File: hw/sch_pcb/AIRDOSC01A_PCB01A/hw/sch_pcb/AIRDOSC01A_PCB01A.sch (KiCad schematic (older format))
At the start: 22 parts, among them J1 HEADER_1x01, J2 HEADER_1x01, J3 HEADER_1x01, J4 HEADER_1x01, J5 CONN_2, J6 CONN_2, J7 HEADER_1x01, M1 HOLE, M2 HOLE, M3 HOLE, M4 HOLE, U1 ARRAYC-60035-4P-BGA, U2 MICROFC-60035-SMT-TR(1), U3 MICROFC-60035-SMT-TR(1)

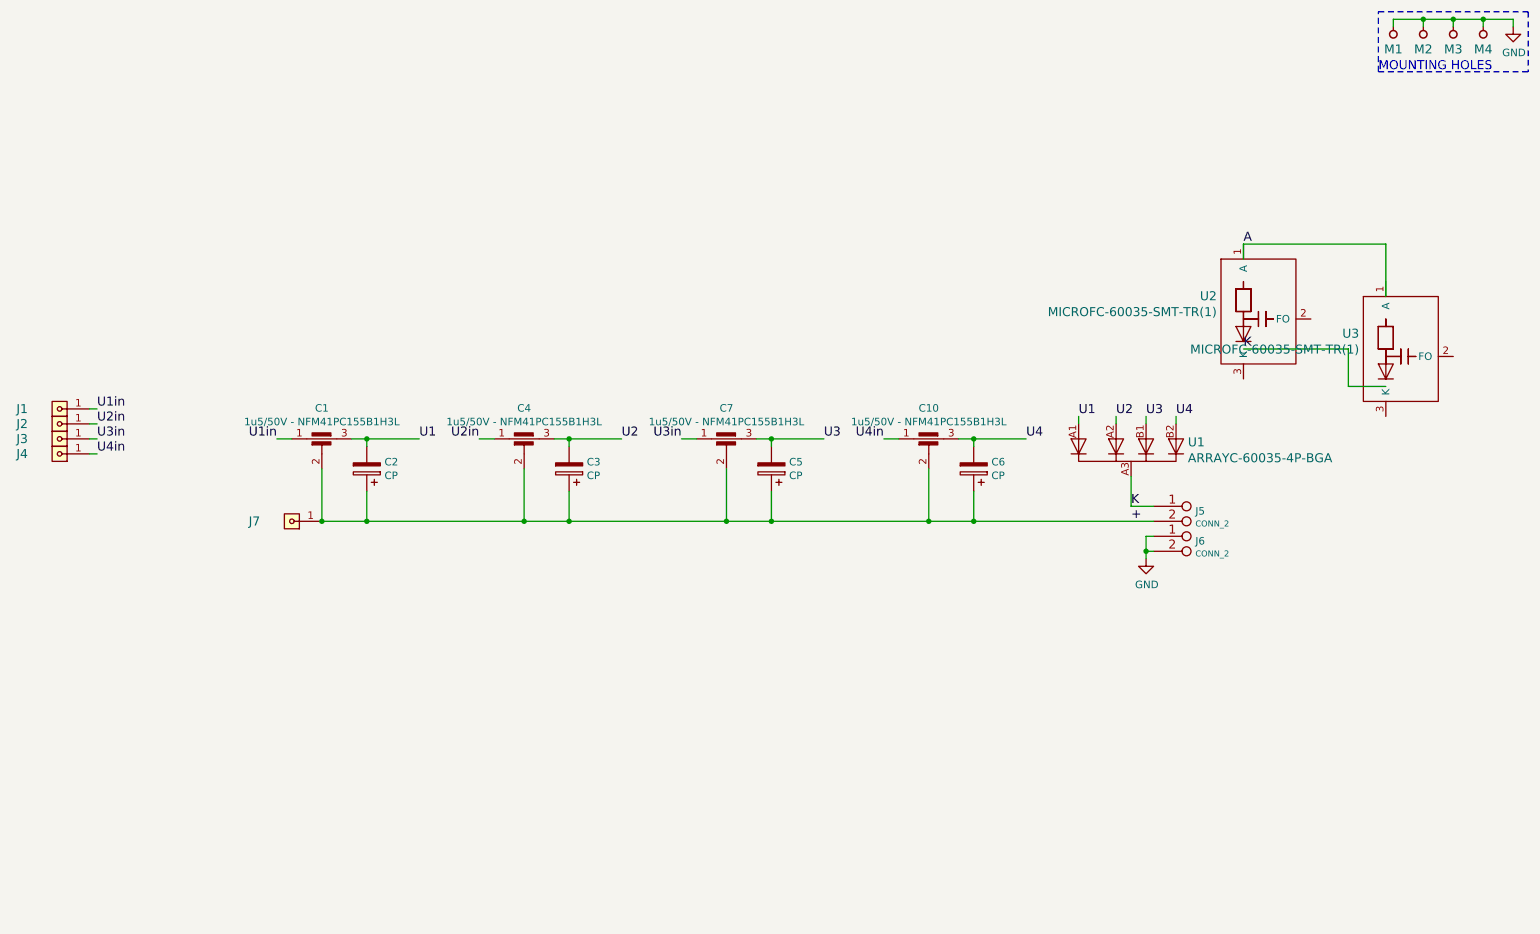
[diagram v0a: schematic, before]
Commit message: edit
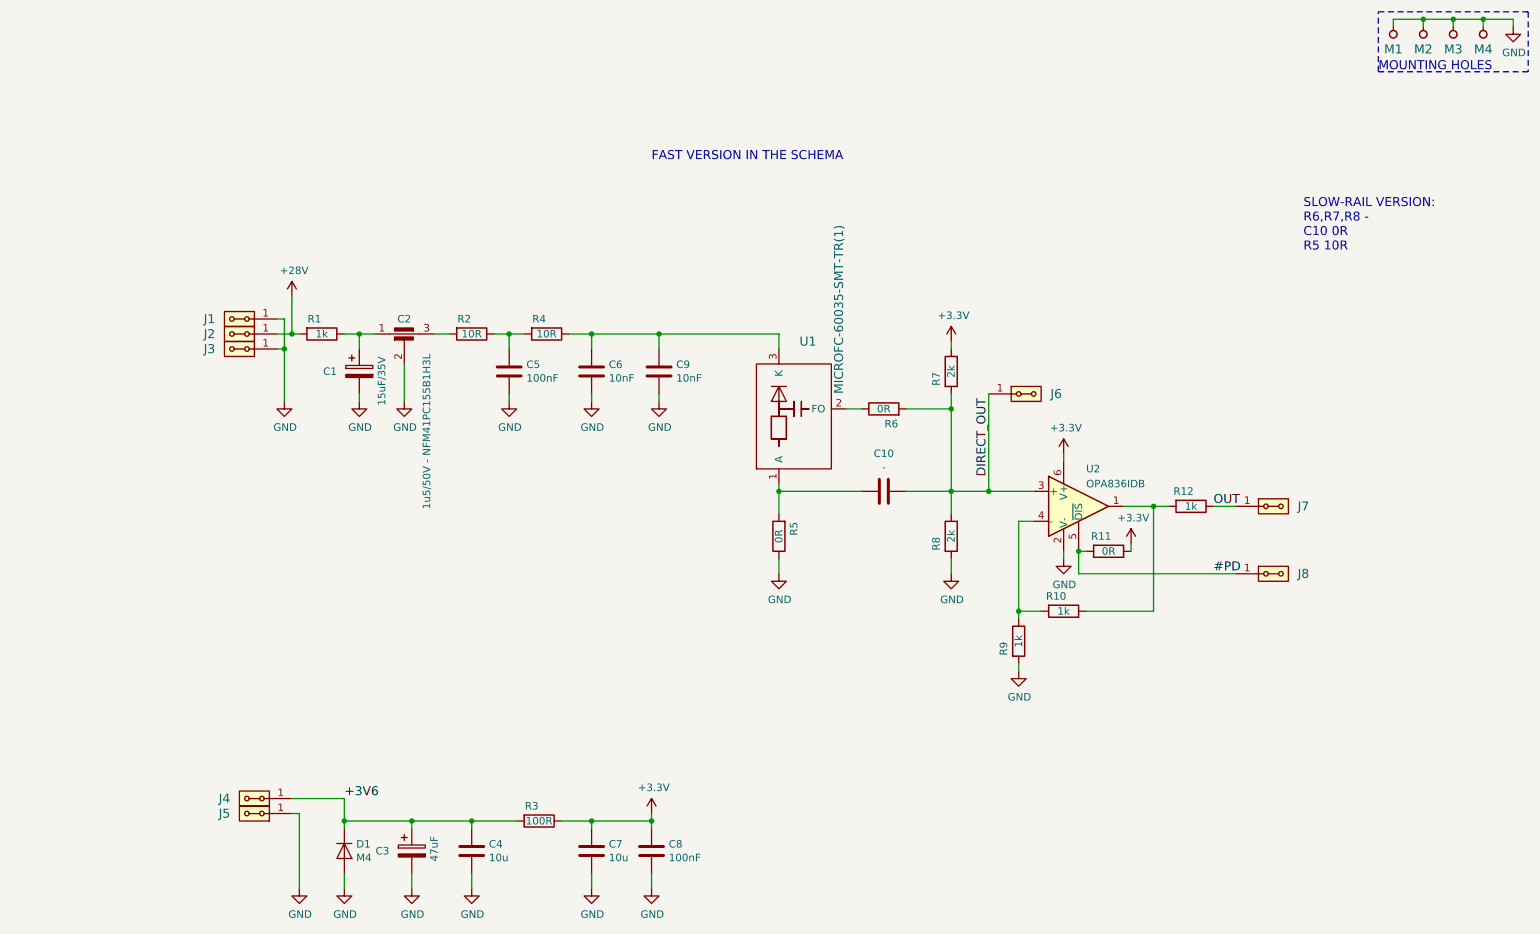
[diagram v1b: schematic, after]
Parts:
- removed C10, C4, C7: 1u5/50V - NFM41PC155B1H3L, Mlab_L:FIR_1806, symbol Device:EMI_Filter_C
- removed C5, C6: CP, Mlab_C:TantalC_SizeC_Reflow, symbol Device:CP
- removed J1, J2, J3, J4, J7: HEADER_1x01, Mlab_Pin_Headers:Straight_1x01, symbol MLAB_HEADER:HEADER_1x01
- removed J5, J6: CONN_2, Mlab_Pin_Headers:SMD_1_2_4x2, symbol MLAB_Jumpers:CONN_2
- removed U1: ARRAYC-60035-4P-BGA, Mlab_D:ArrayC-60035-4P-BGA, symbol MLAB_IO:ARRAYC-60035-4P-BGA
- removed U3: MICROFC-60035-SMT-TR(1), Mlab_IO:MicroFC−60035−SMT, symbol MLAB_IO:MICROFC-60035-SMT-TR(1)
- added C10: -, symbol Device:C
- added C4, C7: 10u, symbol Device:C
- added C5, C8: 100nF, symbol Device:C
- added C6, C9: 10nF, symbol Device:C
- added D1: M4, symbol Device:D
- added J1, J2, J3, J4, J5, J6, J7, J8: HEADER_2x01_PARALLEL, symbol MLAB_HEADER:HEADER_2x01_PARALLEL
- added R1, R10, R12, R9: 1k, symbol Device:R
- added R11, R5, R6: 0R, symbol Device:R
- added R2, R4: 10R, symbol Device:R
- added R3: 100R, symbol Device:R
- added R7, R8: 2k, symbol Device:R
- added U2: OPA836IDB, Package_TO_SOT_SMD:SOT-23-6, symbol Amplifier_Operational:OPA847xDBV
- C1: renamed from C2; value CP -> 15uF/35V
- C3: value CP -> 47uF
- renumbered C1 to C2, U2 to U1
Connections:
- net labels added: #PD, +28V, +3.3V, +3V6, DIRECT_OUT, OUT
- net labels removed: +, A, K, U1, U1in, U2, U2in, U3, U3in, U4, U4in
- wire segments 61 -> 85
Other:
- note added: "FAST VERSION IN THE SCHEMA"
- note added: "SLOW-RAIL VERSION:\nR6,R7,R8 -\nC10 0R\nR5 10R\n\n"
- moved on the sheet: C1, C2, U1

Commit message: edit
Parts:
- C10, C4, C5, C6, C7, C8, C9, R1, R10, R11, R12, R2, R3, R4, R5, R6, R7, R8, R9: footprint (none) -> Mlab_R:SMD-0805
- D1: footprint (none) -> Mlab_D:Diode-SMA_Standard
- J1, J2, J3, J4, J5, J6, J7, J8: footprint (none) -> Mlab_Pin_Headers:Straight_2x01
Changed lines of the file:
@@
 F 0 "R1" V 2950 2650 50  0000 C CNN
 F 1 "1k" V 3050 2700 50  0000 C CNN
-F 2 "" V 2980 2700 50  0001 C CNN
+F 2 "Mlab_R:SMD-0805" V 2980 2700 50  0001 C CNN
 F 3 "~" H 3050 2700 50  0001 C CNN
 	1    3050 2700
@@
 F 0 "R2" V 3950 2650 50  0000 C CNN
 F 1 "10R" V 4050 2700 50  0000 C CNN
-F 2 "" V 3980 2700 50  0001 C CNN
+F 2 "Mlab_R:SMD-0805" V 3980 2700 50  0001 C CNN
 F 3 "~" H 4050 2700 50  0001 C CNN
 	1    4050 2700
@@
 F 0 "C5" H 4415 2996 50  0000 L CNN
 F 1 "100nF" H 4415 2905 50  0000 L CNN
-F 2 "" H 4338 2800 50  0001 C CNN
+F 2 "Mlab_R:SMD-0805" H 4338 2800 50  0001 C CNN
 F 3 "~" H 4300 2950 50  0001 C CNN
 	1    4300 2950
@@
 F 0 "R4" V 4450 2650 50  0000 C CNN
 F 1 "10R" V 4550 2700 50  0000 C CNN
-F 2 "" V 4480 2700 50  0001 C CNN
+F 2 "Mlab_R:SMD-0805" V 4480 2700 50  0001 C CNN
 F 3 "~" H 4550 2700 50  0001 C CNN
 	1    4550 2700
@@
 F 0 "C6" H 4965 2996 50  0000 L CNN
 F 1 "10nF" H 4965 2905 50  0000 L CNN
-F 2 "" H 4888 2800 50  0001 C CNN
+F 2 "Mlab_R:SMD-0805" H 4888 2800 50  0001 C CNN
 F 3 "~" H 4850 2950 50  0001 C CNN
 	1    4850 2950
@@
 F 0 "C9" H 5415 2996 50  0000 L CNN
 F 1 "10nF" H 5415 2905 50  0000 L CNN
-F 2 "" H 5338 2800 50  0001 C CNN
+F 2 "Mlab_R:SMD-0805" H 5338 2800 50  0001 C CNN
 F 3 "~" H 5300 2950 50  0001 C CNN
 	1    5300 2950
@@
 F 0 "R5" V 6000 4000 50  0000 C CNN
 F 1 "0R" V 6100 4050 50  0000 C CNN
-F 2 "" V 6030 4050 50  0001 C CNN
+F 2 "Mlab_R:SMD-0805" V 6030 4050 50  0001 C CNN
 F 3 "~" H 6100 4050 50  0001 C CNN
 	1    6100 4050
@@
 F 0 "R6" V 6700 3150 50  0000 C CNN
 F 1 "0R" V 6800 3200 50  0000 C CNN
-F 2 "" V 6730 3200 50  0001 C CNN
+F 2 "Mlab_R:SMD-0805" V 6730 3200 50  0001 C CNN
 F 3 "~" H 6800 3200 50  0001 C CNN
 	1    6800 3200
@@
 F 0 "R7" V 7150 2900 50  0000 C CNN
 F 1 "2k" V 7250 2950 50  0000 C CNN
-F 2 "" V 7180 2950 50  0001 C CNN
+F 2 "Mlab_R:SMD-0805" V 7180 2950 50  0001 C CNN
 F 3 "~" H 7250 2950 50  0001 C CNN
 	1    7250 2950
@@
 F 0 "R8" V 7150 4000 50  0000 C CNN
 F 1 "2k" V 7250 4050 50  0000 C CNN
-F 2 "" V 7180 4050 50  0001 C CNN
+F 2 "Mlab_R:SMD-0805" V 7180 4050 50  0001 C CNN
 F 3 "~" H 7250 4050 50  0001 C CNN
 	1    7250 4050
@@
 F 0 "C10" V 6548 3750 50  0000 C CNN
 F 1 "-" V 6639 3750 50  0000 C CNN
-F 2 "" H 6838 3600 50  0001 C CNN
+F 2 "Mlab_R:SMD-0805" H 6838 3600 50  0001 C CNN
 F 3 "~" H 6800 3750 50  0001 C CNN
 	1    6800 3750
@@
 F 0 "R9" V 7600 4700 50  0000 C CNN
 F 1 "1k" V 7700 4750 50  0000 C CNN
-F 2 "" V 7630 4750 50  0001 C CNN
+F 2 "Mlab_R:SMD-0805" V 7630 4750 50  0001 C CNN
 F 3 "~" H 7700 4750 50  0001 C CNN
 	1    7700 4750
@@
 F 0 "R11" V 8200 4100 50  0000 C CNN
 F 1 "0R" V 8300 4150 50  0000 C CNN
-F 2 "" V 8230 4150 50  0001 C CNN
+F 2 "Mlab_R:SMD-0805" V 8230 4150 50  0001 C CNN
 F 3 "~" H 8300 4150 50  0001 C CNN
 	1    8300 4150
@@
 F 0 "R10" V 7900 4500 50  0000 C CNN
 F 1 "1k" V 8000 4550 50  0000 C CNN
-F 2 "" V 7930 4550 50  0001 C CNN
+F 2 "Mlab_R:SMD-0805" V 7930 4550 50  0001 C CNN
 F 3 "~" H 8000 4550 50  0001 C CNN
 	1    8000 4550
@@
 F 0 "R12" V 8750 3800 50  0000 C CNN
 F 1 "1k" V 8850 3850 50  0000 C CNN
-F 2 "" V 8780 3850 50  0001 C CNN
+F 2 "Mlab_R:SMD-0805" V 8780 3850 50  0001 C CNN
 F 3 "~" H 8850 3850 50  0001 C CNN
 	1    8850 3850
@@
 F 0 "C4" H 4165 6196 50  0000 L CNN
 F 1 "10u" H 4165 6105 50  0000 L CNN
-F 2 "" H 4088 6000 50  0001 C CNN
+F 2 "Mlab_R:SMD-0805" H 4088 6000 50  0001 C CNN
 F 3 "~" H 4050 6150 50  0001 C CNN
 	1    4050 6150
@@
 F 0 "C8" H 5365 6196 50  0000 L CNN
 F 1 "100nF" H 5365 6105 50  0000 L CNN
-F 2 "" H 5288 6000 50  0001 C CNN
+F 2 "Mlab_R:SMD-0805" H 5288 6000 50  0001 C CNN
 F 3 "~" H 5250 6150 50  0001 C CNN
 	1    5250 6150
@@
 F 0 "C7" H 4965 6196 50  0000 L CNN
 F 1 "10u" H 4965 6105 50  0000 L CNN
-F 2 "" H 4888 6000 50  0001 C CNN
+F 2 "Mlab_R:SMD-0805" H 4888 6000 50  0001 C CNN
 F 3 "~" H 4850 6150 50  0001 C CNN
 	1    4850 6150
@@
 F 0 "R3" V 4400 5900 50  0000 C CNN
 F 1 "100R" V 4500 5950 50  0000 C CNN
-F 2 "" V 4430 5950 50  0001 C CNN
+F 2 "Mlab_R:SMD-0805" V 4430 5950 50  0001 C CNN
 F 3 "~" H 4500 5950 50  0001 C CNN
 	1    4500 5950
@@
 F 0 "J7" H 9600 3850 60  0000 C CNN
 F 1 "HEADER_2x01_PARALLEL" H 9318 3991 60  0001 C CNN
-F 2 "" H 9400 3850 60  0000 C CNN
+F 2 "Mlab_Pin_Headers:Straight_2x01" H 9400 3850 60  0001 C CNN
 F 3 "" H 9400 3850 60  0000 C CNN
 	1    9400 3850
@@
 F 0 "J8" H 9600 4300 60  0000 C CNN
 F 1 "HEADER_2x01_PARALLEL" H 9318 4441 60  0001 C CNN
-F 2 "" H 9400 4300 60  0000 C CNN
+F 2 "Mlab_Pin_Headers:Straight_2x01" H 9400 4300 60  0001 C CNN
 F 3 "" H 9400 4300 60  0000 C CNN
 	1    9400 4300
@@
 F 0 "J6" H 7950 3100 60  0000 C CNN
 F 1 "HEADER_2x01_PARALLEL" H 7668 3241 60  0001 C CNN
-F 2 "" H 7750 3100 60  0000 C CNN
+F 2 "Mlab_Pin_Headers:Straight_2x01" H 7750 3100 60  0001 C CNN
 F 3 "" H 7750 3100 60  0000 C CNN
 	1    7750 3100
@@
 F 0 "D1" V 3154 6229 50  0000 L CNN
 F 1 "M4" V 3245 6229 50  0000 L CNN
-F 2 "" H 3200 6150 50  0001 C CNN
+F 2 "Mlab_D:Diode-SMA_Standard" H 3200 6150 50  0001 C CNN
 F 3 "~" H 3200 6150 50  0001 C CNN
 	1    3200 6150
@@
 F 0 "J4" H 2800 5800 60  0000 C CNN
 F 1 "HEADER_2x01_PARALLEL" H 2518 5941 60  0001 C CNN
-F 2 "" H 2600 5800 60  0000 C CNN
+F 2 "Mlab_Pin_Headers:Straight_2x01" H 2600 5800 60  0001 C CNN
 F 3 "" H 2600 5800 60  0000 C CNN
 	1    2600 5800
@@
 F 0 "J5" H 2800 5900 60  0000 C CNN
 F 1 "HEADER_2x01_PARALLEL" H 2518 6041 60  0001 C CNN
-F 2 "" H 2600 5900 60  0000 C CNN
+F 2 "Mlab_Pin_Headers:Straight_2x01" H 2600 5900 60  0001 C CNN
 F 3 "" H 2600 5900 60  0000 C CNN
 	1    2600 5900
@@
 F 0 "J2" H 2700 2700 60  0000 C CNN
 F 1 "HEADER_2x01_PARALLEL" H 2418 2841 60  0001 C CNN
-F 2 "" H 2500 2700 60  0000 C CNN
+F 2 "Mlab_Pin_Headers:Straight_2x01" H 2500 2700 60  0001 C CNN
 F 3 "" H 2500 2700 60  0000 C CNN
 	1    2500 2700
@@
 F 0 "J3" H 2700 2800 60  0000 C CNN
 F 1 "HEADER_2x01_PARALLEL" H 2418 2941 60  0001 C CNN
-F 2 "" H 2500 2800 60  0000 C CNN
+F 2 "Mlab_Pin_Headers:Straight_2x01" H 2500 2800 60  0001 C CNN
 F 3 "" H 2500 2800 60  0000 C CNN
 	1    2500 2800
@@
 F 0 "J1" H 2700 2600 60  0000 C CNN
 F 1 "HEADER_2x01_PARALLEL" H 2418 2741 60  0001 C CNN
-F 2 "" H 2500 2600 60  0000 C CNN
+F 2 "Mlab_Pin_Headers:Straight_2x01" H 2500 2600 60  0001 C CNN
 F 3 "" H 2500 2600 60  0000 C CNN
 	1    2500 2600
